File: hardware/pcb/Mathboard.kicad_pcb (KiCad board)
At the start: 4 copper layers, 95.6 x 73.6 mm, 93 parts, among them J3 TYPE-C sinking plate, Q1 2N7002VC-, Q2 2N7002VC-, SW1 SW_Push, SW10 SW_Push, SW11 SW_Push, SW12 SW_Push, SW13 SW_Push, SW14 SW_Push, SW15 SW_Push, SW16 SW_Push, SW17 MSK13C02, SW18 SWITCH, SW2 SW_Push, SW3 SW_Push, SW4 SW_Push, SW5 SW_Push, SW6 SW_Push, SW7 SW_Push, SW8 SW_Push, SW9 SW_Push, U1 W25Q64JV, U3 USBLC6-2P6, U4 XC6206P332MR-G, U5 PSSI2021SAY, U6 RP2040, U7 74LVC1T45, Y1 12MHz

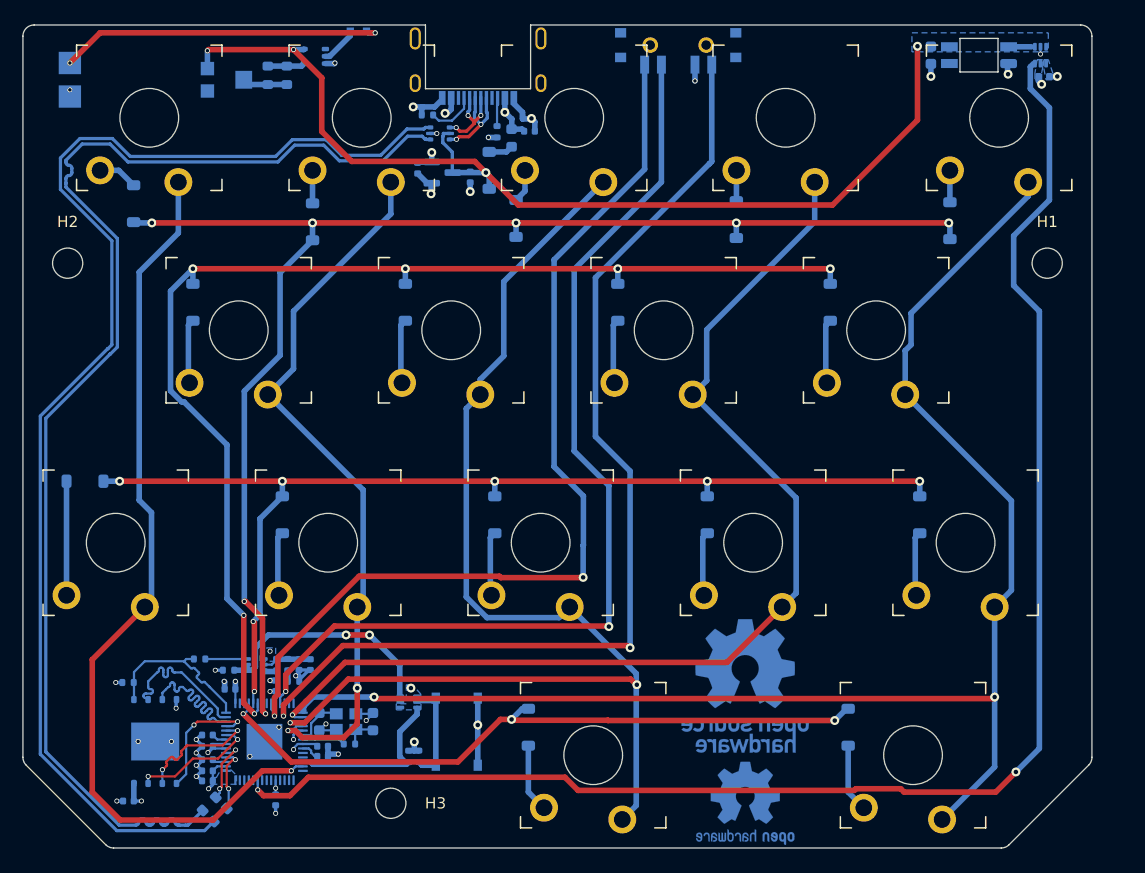
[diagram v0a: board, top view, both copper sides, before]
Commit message: Revision 4
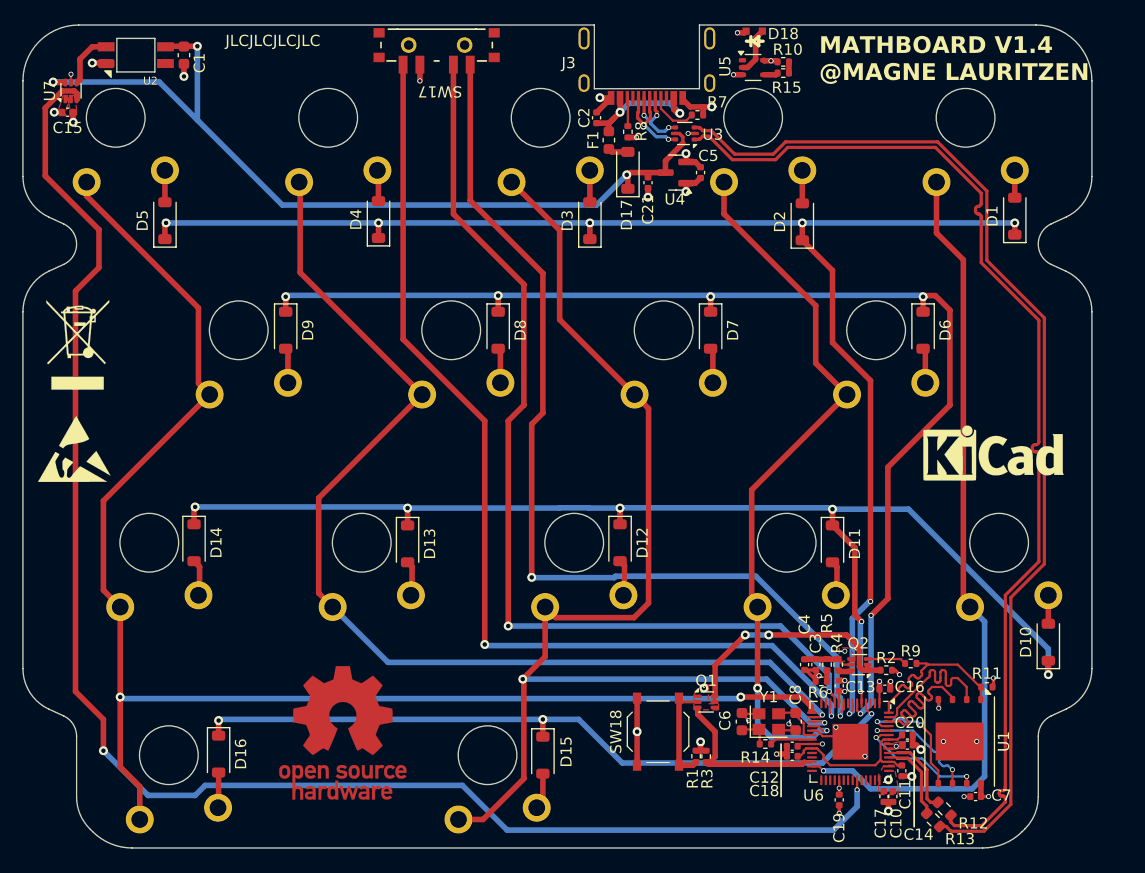
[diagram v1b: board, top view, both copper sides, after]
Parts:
- removed H1, H2, H3: MountingHole, MountingHole:MountingHole_2.7mm
- removed the REF** at (148.6, 112.3) (x2)
- removed RV1: 20k, Potentiometer_SMD:Potentiometer_Bourns_TC33X_Vertical
- removed TP1, TP2: TestPoint, TestPoint:TestPoint_Pad_2.0x2.0mm
- added REF**: WEEE-Logo_5.6x8mm_SilkScreen, Symbol:WEEE-Logo_5.6x8mm_SilkScreen, F.Cu at (88.9, 71.3)
- added REF**: ESD-Logo_6.6x6mm_SilkScreen, Symbol:ESD-Logo_6.6x6mm_SilkScreen, F.Cu at (88.6, 80.6)
- added REF**: KiCad-Logo_5mm_SilkScreen, Symbol:KiCad-Logo_5mm_SilkScreen, F.Cu at (170.8, 81.5)
- C1, C10, C11, C12, C13, C14, C15, C16, C17, C18, C19, C2, C20, C21, C3, C4, C5, C6, C7, C8, D1, D10, D11, D12, D13, D14, D15, D16, D17, D18, D2, D3, D4, D5, D6, D7, D8, D9, F1, J3, Q1, Q2, R1, R11, R12, R13, R14, R2, R3, R4, R5, R6, R7, R8, R9, REF** (x2), SW17, SW18, U2, U3, U4, U5, U6, U7, Y1: moved to F.Cu
- R10, R15: value 27 -> 10k; footprint Resistor_SMD:R_0603_1608Metric -> Resistor_SMD:R_0402_1005Metric; moved to F.Cu
- SW1, SW10, SW11, SW12, SW13, SW14, SW15, SW16, SW2, SW3, SW4, SW5, SW6, SW7, SW8, SW9: moved to B.Cu
- U1: footprint Package_SON:WSON-8-1EP_8x6mm_P1.27mm_EP3.4x4.3mm -> mathboard:WSON-8-1EP_8x6mm_P1.27mm_EP3.4x4.3mm; moved to F.Cu
- moved C15 87.4 mm to (88.0, 50.5), turned to 0 degrees
- moved D10 87.3 mm to (175.7, 97.9), turned to 90 degrees
- moved U7 86.8 mm to (88.3, 48.6)
- moved SW10 79.0 mm to (171.3, 89.0), turned to 180 degrees
- moved SW5 79.0 mm to (92.3, 51.0), turned to 180 degrees
- moved D1 78.8 mm to (172.7, 59.8)
- moved R11 76.8 mm to (170.2, 101.9), turned to 180 degrees
- moved C7 75.8 mm to (169.2, 111.7)
- moved U2 75.4 mm to (94.1, 45.4), turned to 180 degrees
- moved SW1 73.0 mm to (168.3, 51.0), turned to 180 degrees
- moved SW14 73.0 mm to (95.3, 89.0), turned to 180 degrees
- moved U1 71.9 mm to (167.8, 106.8)
- moved D5 70.2 mm to (96.7, 60.2)
- moved C1 66.8 mm to (98.4, 45.4)
- moved SW16 66.5 mm to (97.0, 108.0), turned to 180 degrees
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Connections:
- D18 pad 2: Net-(D18-A) -> GND
- R10 pad 1: Net-(R10-Pad1) -> +3V3
- R15 pad 1: Net-(R10-Pad1) -> Net-(R10-Pad2)
- R15 pad 2: Net-(R10-Pad2) -> Net-(R15-Pad2)
- U5 pad 4: Net-(R10-Pad1) -> Net-(R15-Pad2)
- U5 pad 5: +5V -> +3V3
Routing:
- net Net-(D18-A): track 29.3 -> 0.00 mm, vias 2 -> 0
- net /Microcontroller/USB+: track 113.4 -> 95.0 mm
- net /Microcontroller/USB-: track 113.3 -> 95.2 mm
- net +5V: track 93.5 -> 77.0 mm, vias 4 -> 3
- net +1V1: track 4.29 -> 14.7 mm
- net ROW2: track 98.1 -> 108.3 mm
- net COL0: track 80.5 -> 71.7 mm
- net Net-(D10-A): track 10.2 -> 2.55 mm
- net +3V3: track 22.9 -> 17.7 mm, vias 13 -> 14
- net ROW3: track 61.0 -> 66.0 mm
- net ROW0: track 125.4 -> 129.6 mm
- net Net-(R10-Pad1): track 3.34 -> 0.00 mm
- net Net-(R10-Pad2): track 4.03 -> 1.00 mm
- net Net-(D16-A): track 6.13 -> 3.17 mm
- net Net-(D15-A): track 6.13 -> 3.28 mm
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- added copper zone on F.Cu, net +3V3
- added copper zone on In2.Cu, net +3V3
- added copper zone on F.Cu, net GND
- added copper zone on In1.Cu, net GND
- removed copper zone on B.Cu, net +3V3
- removed copper zone on In1.Cu, net +3V3
- removed copper zone on B.Cu, net +5V
- removed copper zone on B.Cu, net GND
- removed copper zone on In2.Cu, net GND
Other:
- outline, holes or cut-outs redrawn
- board text added: "MATHBOARD V1.4 @MAGNE LAURITZEN"
- board text removed: "GND"
- board text removed: "LED"
- board text removed: "MATHBOARD V1.0 PCB REV 3 MAGNE EIK LAURITZEN"
